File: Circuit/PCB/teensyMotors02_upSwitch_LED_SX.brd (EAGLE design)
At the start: 72 x 150.1 mm, 65 parts, among them SW1 219-10, SW2 B3F-1000, SW3 B3F-1000, SW4 B3F-1000, SW5 B3F-1000, SW6 B3F-1000, SW7 B3F-1000, SW8 B3F-1000, SW9 B3F-1000

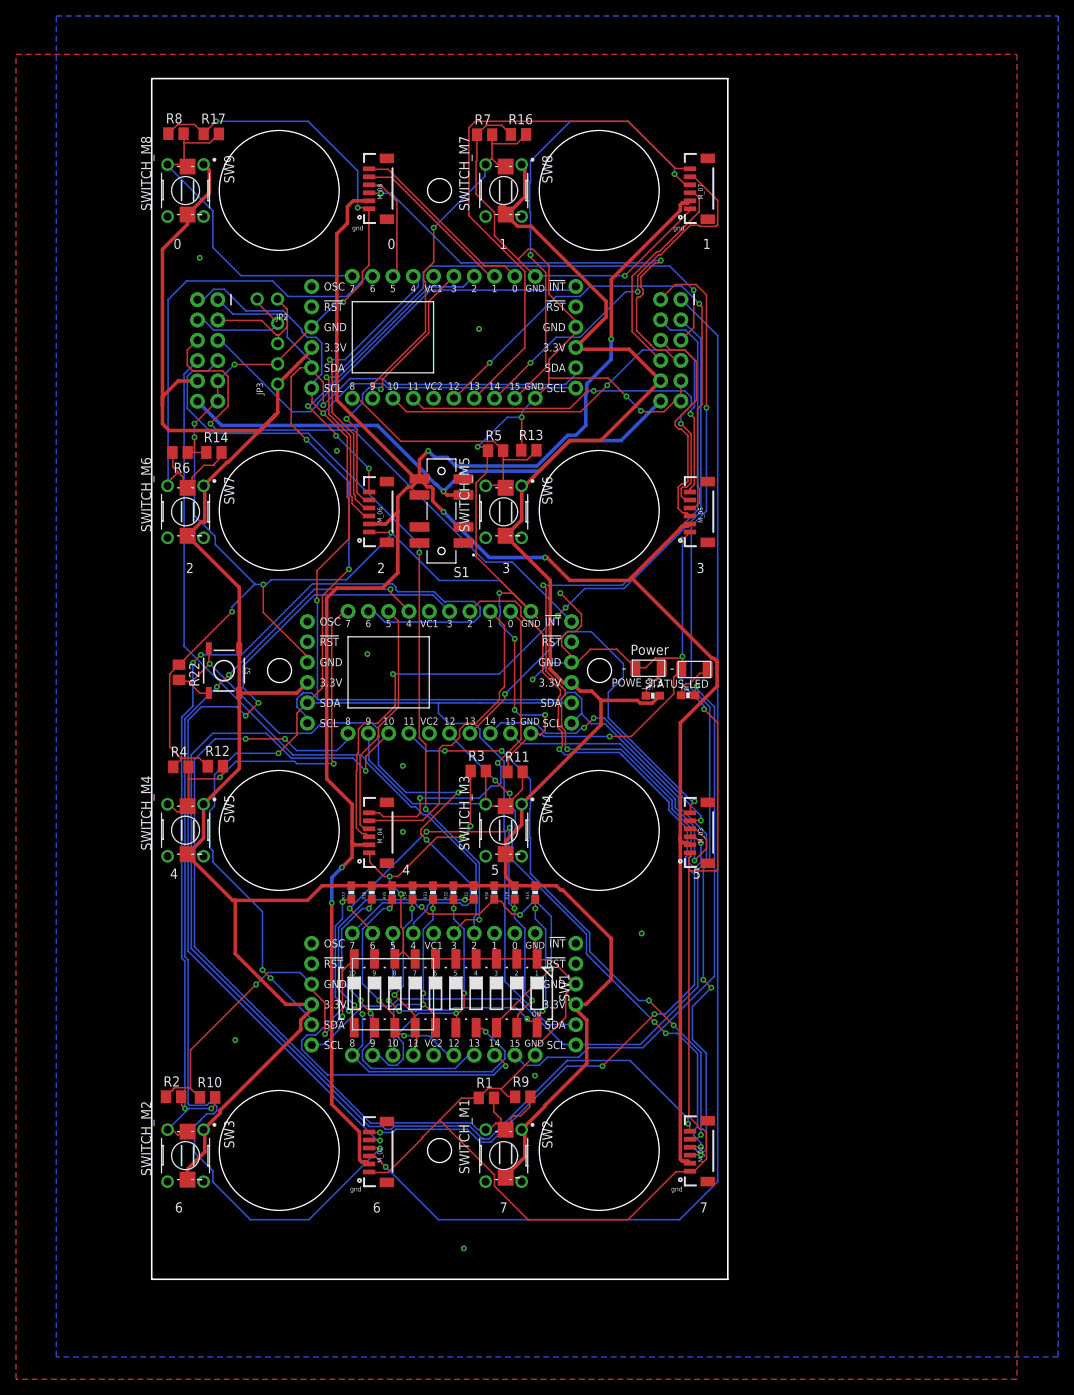
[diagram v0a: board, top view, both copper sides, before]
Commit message: update circuit sx
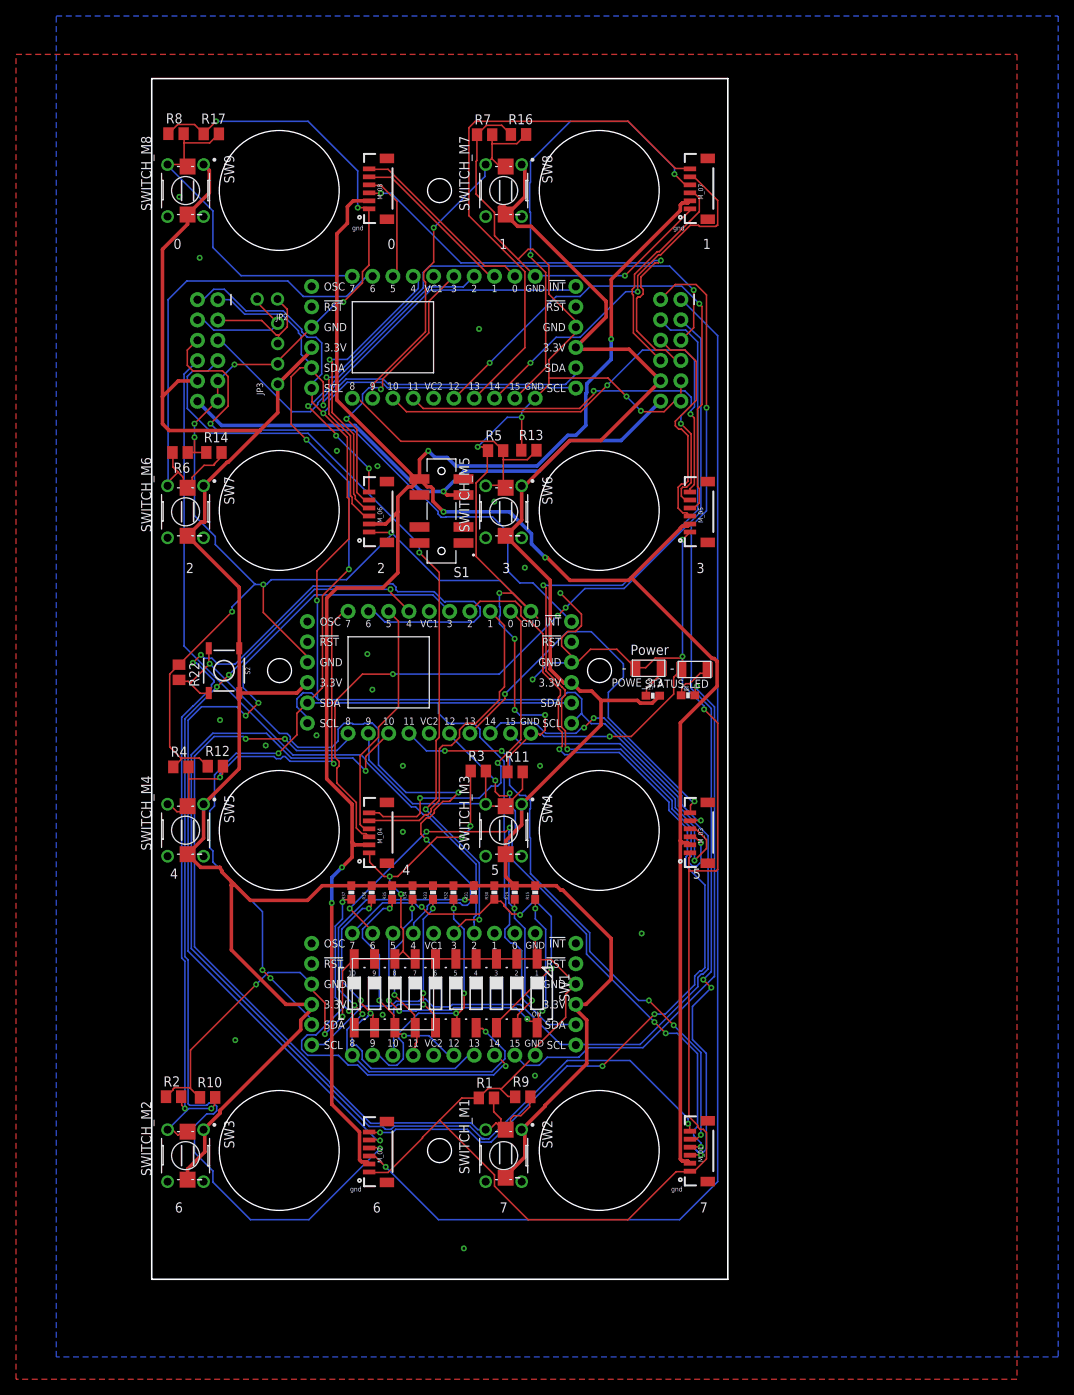
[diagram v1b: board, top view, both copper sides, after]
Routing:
- net NEOPIXEL_04: track 97.0 -> 100.5 mm
- net 6_SX1: track 127.1 -> 130.5 mm
- net 4_SX3: track 79.8 -> 83.0 mm
- net INT_01: track 71.5 -> 74.7 mm
- net 13_SX3: track 41.2 -> 42.7 mm
- net 3_SX3: track 98.7 -> 100.1 mm
- net 12_SX1: track 67.8 -> 69.1 mm
- net 3.3V: track 426.7 -> 425.4 mm
- net 2_SX1: track 118.4 -> 119.6 mm
- net SCL_00: track 243.5 -> 244.6 mm
- net SDA_00: track 245.1 -> 246.1 mm
- net 7_SX1: track 49.2 -> 50.2 mm
- net 8_SX3: track 62.5 -> 63.1 mm
- net 8_SX1: track 105.8 -> 106.3 mm
- net GND_MCU: track 705.0 -> 704.8 mm, vias 41 -> 53

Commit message: return to previous pcb design
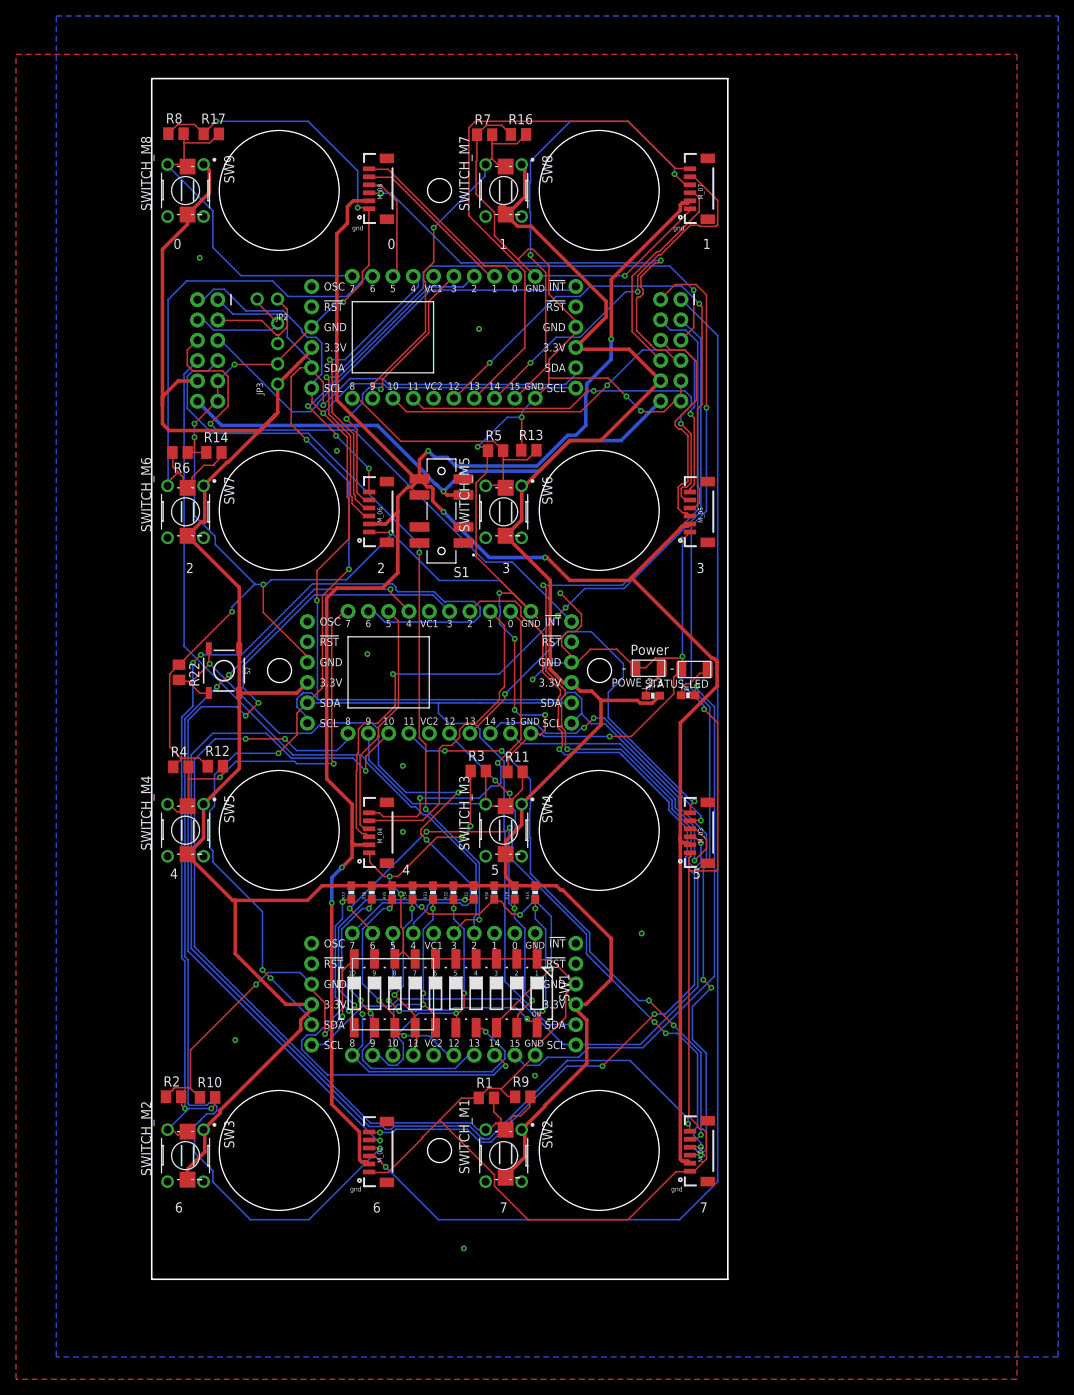
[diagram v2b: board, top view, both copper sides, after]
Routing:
- net NEOPIXEL_04: track 100.5 -> 97.0 mm
- net 6_SX1: track 130.5 -> 127.1 mm
- net 4_SX3: track 83.0 -> 79.8 mm
- net INT_01: track 74.7 -> 71.5 mm
- net 13_SX3: track 42.7 -> 41.2 mm
- net 3_SX3: track 100.1 -> 98.7 mm
- net 12_SX1: track 69.1 -> 67.8 mm
- net 3.3V: track 425.4 -> 426.7 mm
- net 2_SX1: track 119.6 -> 118.4 mm
- net SCL_00: track 244.6 -> 243.5 mm
- net SDA_00: track 246.1 -> 245.1 mm
- net 7_SX1: track 50.2 -> 49.2 mm
- net 8_SX3: track 63.1 -> 62.5 mm
- net 8_SX1: track 106.3 -> 105.8 mm
- net GND_MCU: track 704.8 -> 705.0 mm, vias 53 -> 41
